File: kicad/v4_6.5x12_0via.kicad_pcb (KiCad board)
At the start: 2 copper layers, 33.6 x 17.7 mm, 18 parts, among them J3 FDTI, SW1 SW_Push, U1 ATmega328P-A

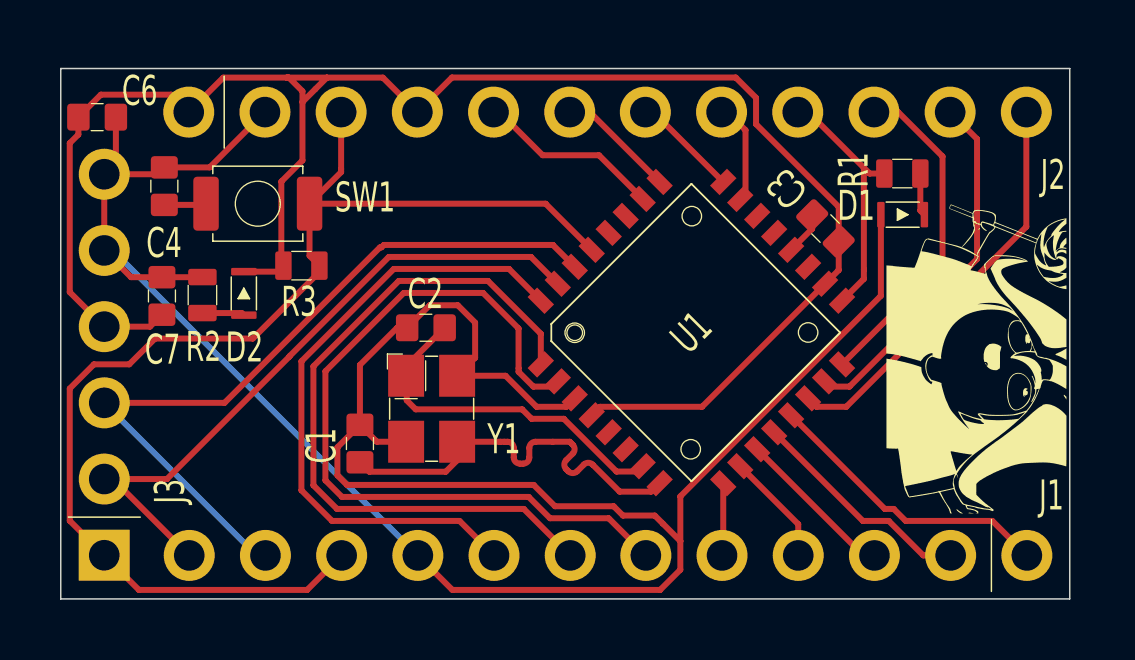
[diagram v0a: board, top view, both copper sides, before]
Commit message: a
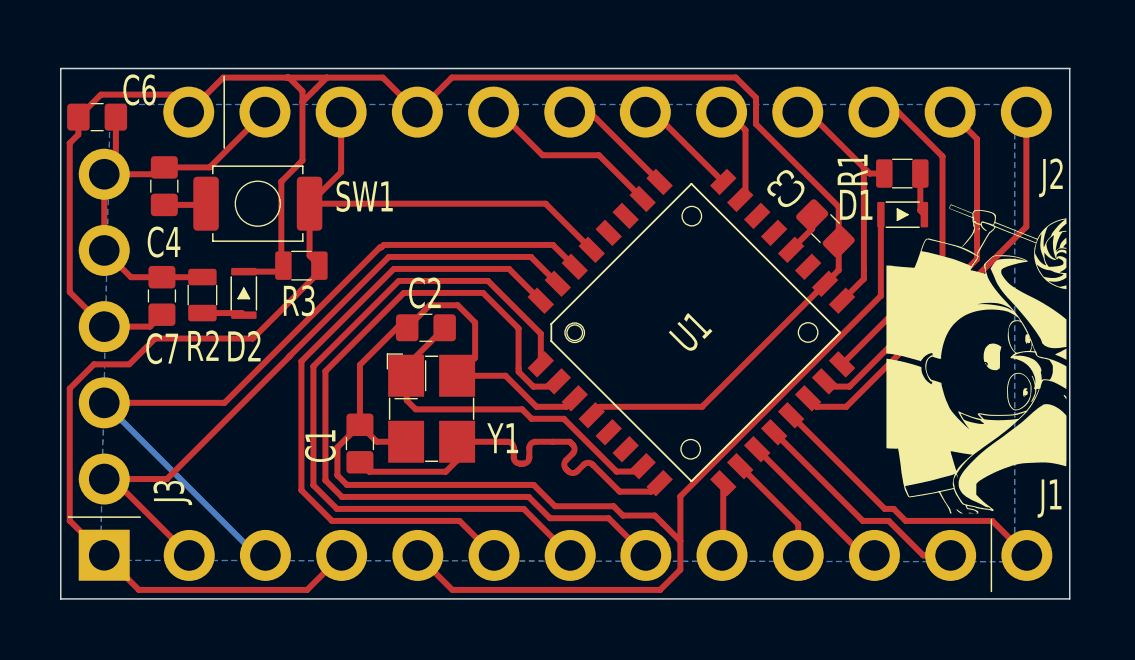
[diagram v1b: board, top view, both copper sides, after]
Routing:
- net GND: track 83.9 -> 69.5 mm
- added copper zone on B.Cu, net GND
